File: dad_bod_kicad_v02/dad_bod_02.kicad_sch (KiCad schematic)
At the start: 65 parts, among them J1 Conn_01x01, J10 Conn_01x03_Male, J12 USB4085-GF-A_REVA4, J13 Conn_01x03_Male, J2 Conn_01x01, J3 Conn_01x01, J4 Conn_01x01, J5 Conn_01x03_Male, J6 Conn_02x15_Odd_Even, J7 BNC5-J-P-GN-RA-BH2D, J8 Conn_01x03_Male, J9 Conn_02x15_Odd_Even, K1 EC2-5NU, K2 EC2-5NU, Q1 2N3904, Q2 2N3904, T1 GT07-110-013, U1 SL1002A600SP

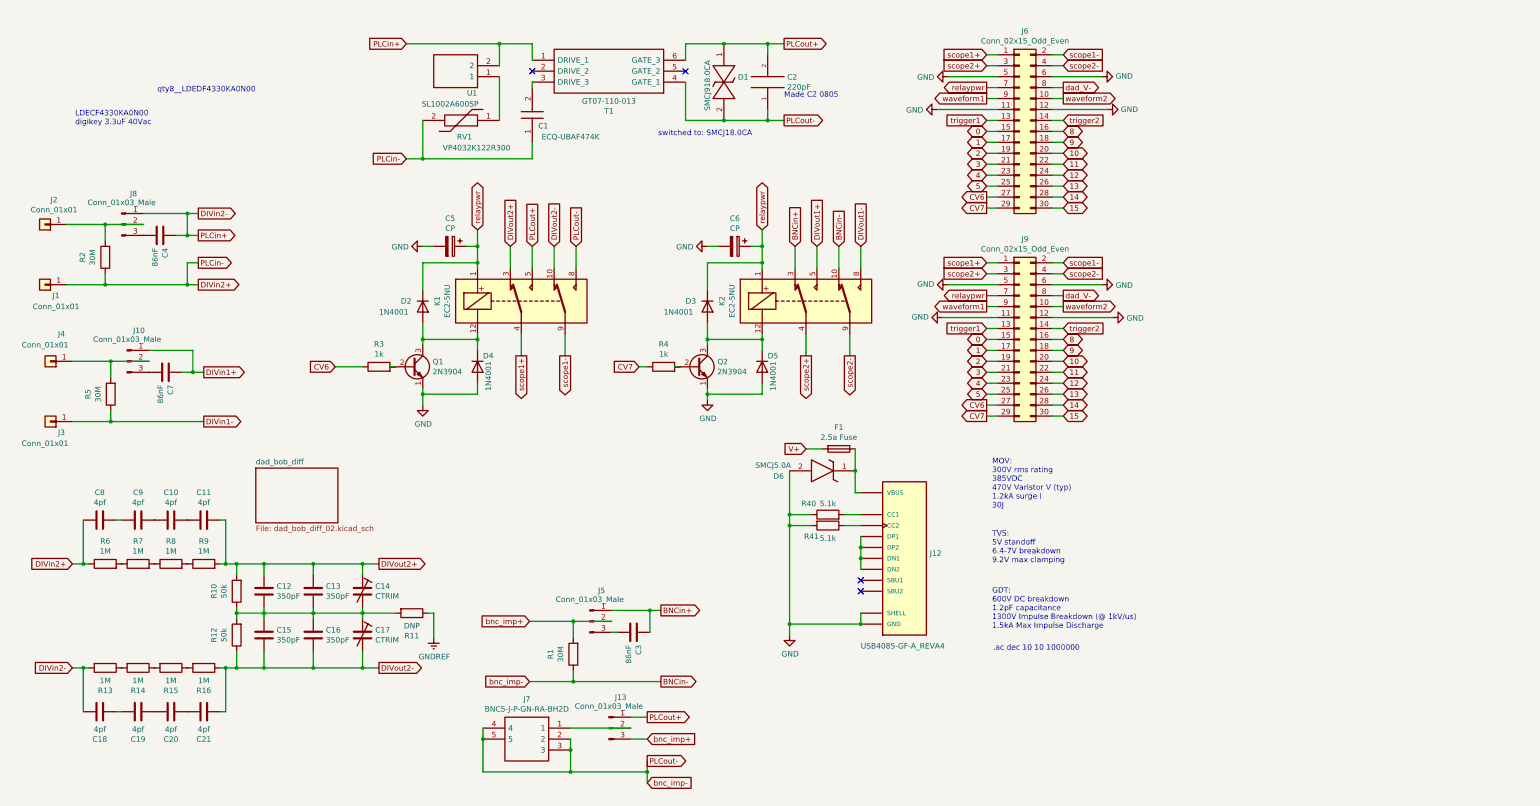
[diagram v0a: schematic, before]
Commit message: Version saving, before rearranging relays
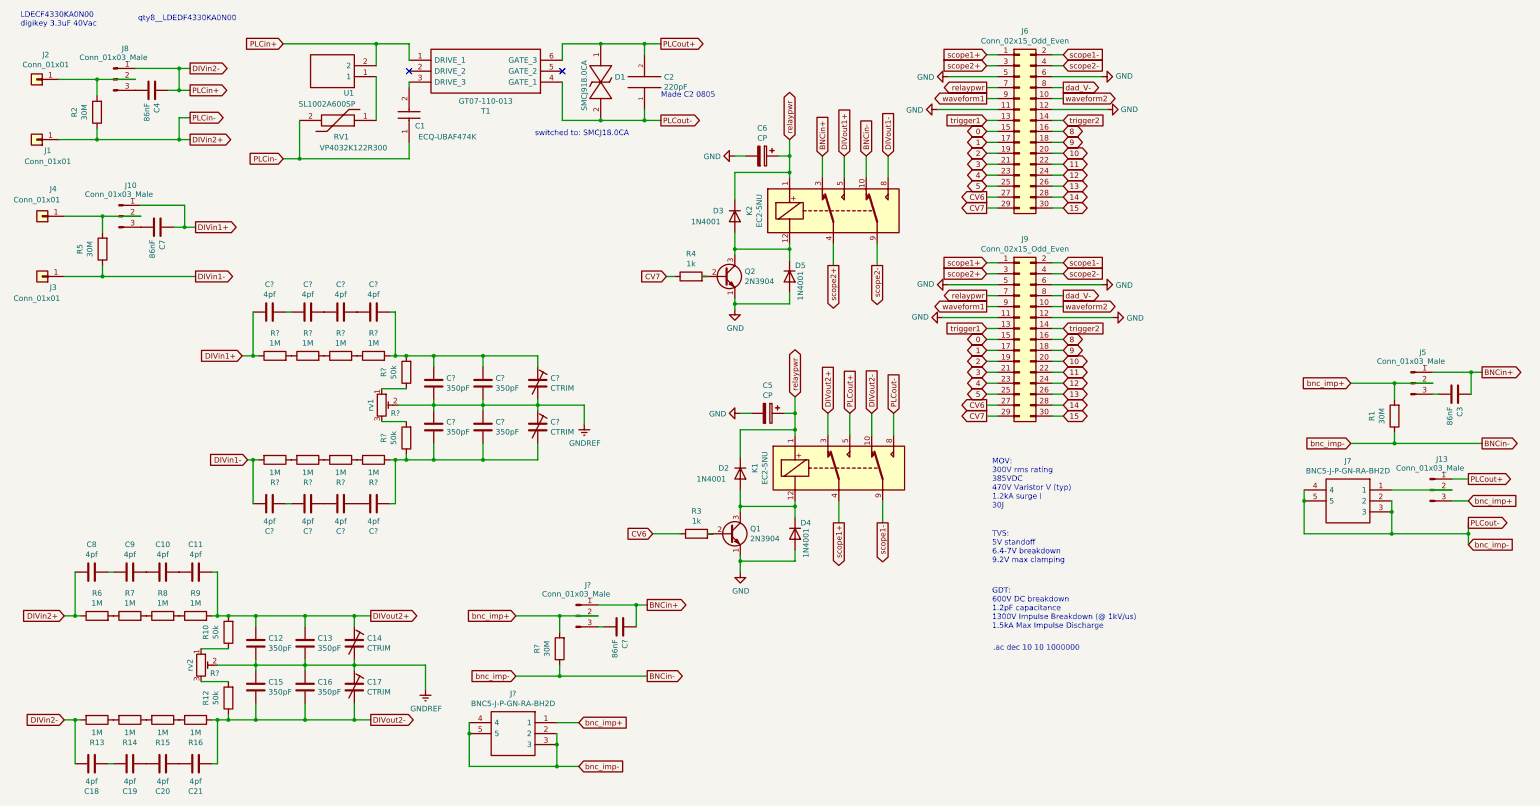
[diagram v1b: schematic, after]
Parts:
- removed D6: SMCJ5.0A, kyuditsky_kicad_fp:littlefuseTVS, symbol dad_bob-rescue:SMCJ5.0A-00_kyuditsky_kicad
- removed F1: 2.5a Fuse, Resistor_THT:R_Axial_DIN0204_L3.6mm_D1.6mm_P2.54mm_Vertical, symbol Device:Fuse
- removed J12: USB4085-GF-A_REVA4, GCT_USB4085-GF-A_REVA4, symbol dad_bob-rescue:USB4085-GF-A_REVA4-00_kyuditsky_kicad
- removed R11: DNP, Resistor_SMD:R_0805_2012Metric_Pad1.15x1.40mm_HandSolder, symbol Device:R
- removed R40, R41: 5.1k, Resistor_SMD:R_0805_2012Metric_Pad1.15x1.40mm_HandSolder, symbol Device:R
- added C? (x8): 4pf, Capacitor_SMD:C_0805_2012Metric_Pad1.15x1.40mm_HandSolder, symbol Device:C
- added C? (x4): 350pF, Capacitor_SMD:C_0805_2012Metric_Pad1.15x1.40mm_HandSolder, symbol Device:C
- added C?: 86nF, Capacitor_SMD:C_0805_2012Metric_Pad1.15x1.40mm_HandSolder, symbol Device:C
- added C? (x2): CTRIM, Capacitor_SMD:C_Trimmer_Voltronics_JQ, symbol dad_bob-rescue:CTRIM-Device
- added J?: Conn_01x03_Male, Connector_PinHeader_2.54mm:PinHeader_1x03_P2.54mm_Vertical, symbol Connector:Conn_01x03_Male
- added J?: BNC5-J-P-GN-RA-BH2D, BNC5-J-P-GN-RA-BH2D_kicad:BNC5JPGNRABH2D, symbol dad_bob-rescue:BNC5-J-P-GN-RA-BH2D-00_kyuditsky_kicad
- added R? (x8): 1M, Resistor_SMD:R_0805_2012Metric_Pad1.15x1.40mm_HandSolder, symbol Device:R
- added R?: 30M, Resistor_SMD:R_0805_2012Metric_Pad1.15x1.40mm_HandSolder, symbol Device:R
- added R? (x2): 50k, Resistor_SMD:R_0805_2012Metric_Pad1.15x1.40mm_HandSolder, symbol Device:R
- added R?: rv1, symbol Device:R_Potentiometer_Trim
- added R?: rv2, symbol Device:R_Potentiometer_Trim
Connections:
- net BNCin+: now also C?.2, J?.1 (Pin_1)
- net BNCin-: now also J?.2, J?.3, J?.4, J?.5, R?.1
- net DIVin1+: now also C?.2, R?.1
- net DIVin1-: now also C?.1, R?.2
- net GNDREF: now also C12.1, C13.1, C14.2, C15.2, C16.2, C17.1, C?.1, C?.1, C?.1, C?.2, C?.2, C?.2, R?.2, R?.2
- net bnc_imp+: now also J?.1, J?.2 (Pin_2), R?.2
- new net: R10.1, R?.1
- new net: R12.2, R?.3
- new net: C?.1, C?.2 (x6)
- new net: R?.1, R?.2 (x6)
- new net: C?.1, J?.3 (Pin_3)
- new net: C?.1, C?.1, C?.2, C?.2, R?.2, R?.2
- new net: C?.1, C?.1, C?.2, C?.2, R?.1, R?.1
- new net: R?.1, R?.1
- new net: R?.2, R?.3
- no-connect marks 4 -> 2
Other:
- removed sheet dad_bob_diff
- moved on the sheet: C1, C10, C11, C12, C13, C14, C15, C16, C17, C18, C19, C2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
